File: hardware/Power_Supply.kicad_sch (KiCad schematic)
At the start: 62 parts, among them IC1 LM13700, IC2 LM13700, IC3 LM13700, J5 USB_B, SW1 POWER, U1 TL064, U19 TL064

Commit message: hardware: LCSC review, production files ok
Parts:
- PS1: LCSC C5198614 -> C512062
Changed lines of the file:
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@@
 			)
 		)
-		(property "LCSC" "C5198614"
+		(property "LCSC" "C512062"
 			(at 82.55 76.2 0)
 			(effects

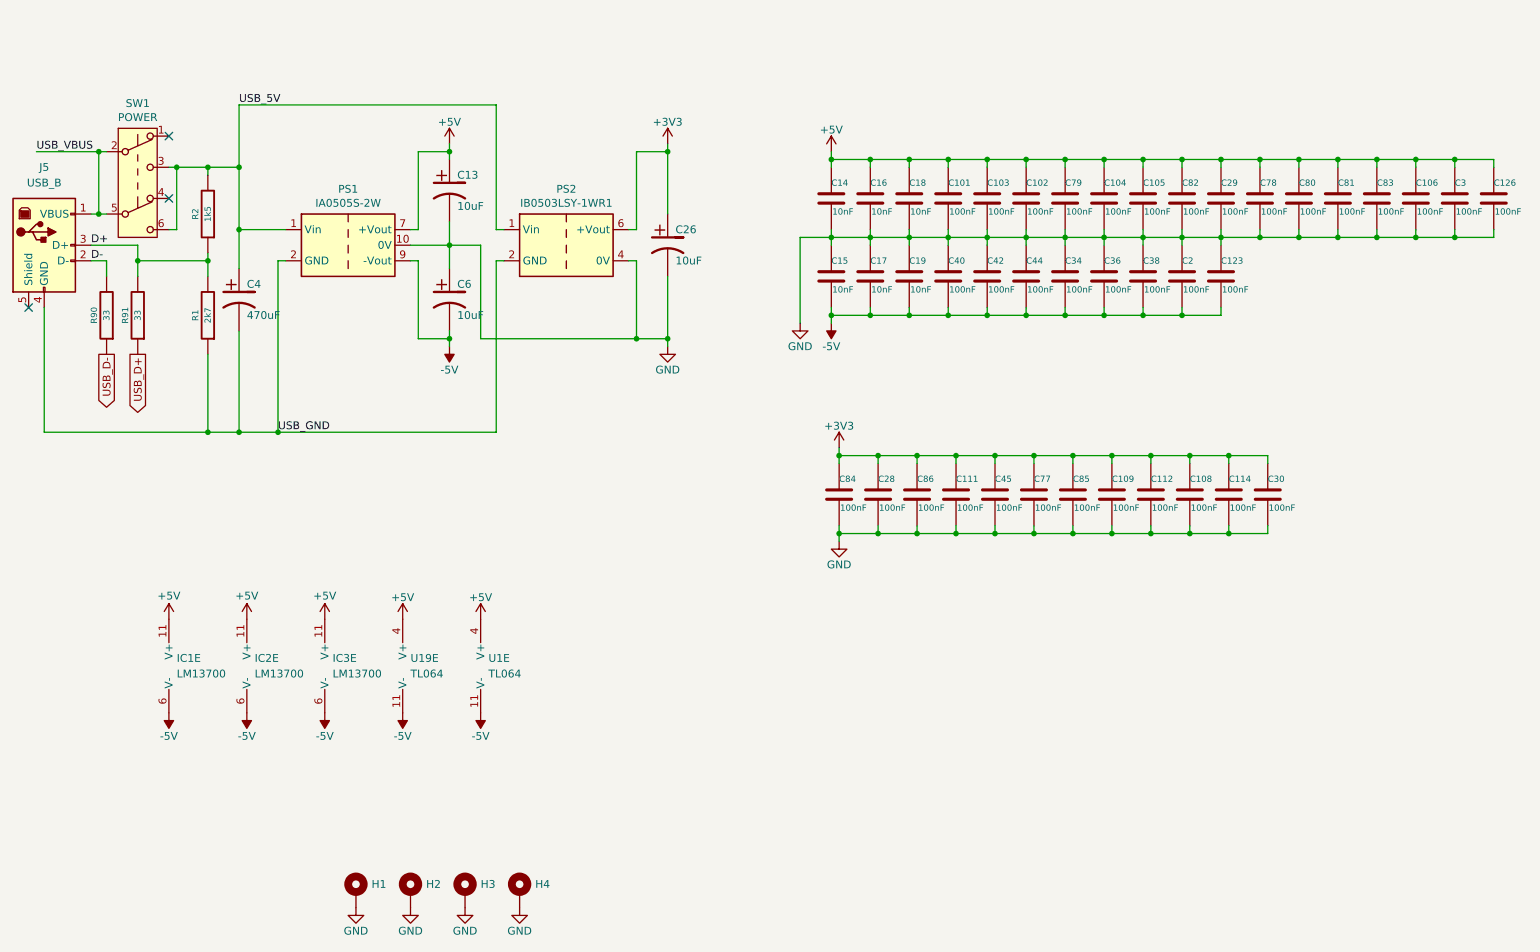
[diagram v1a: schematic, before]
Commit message: hardware: sch/pcb changes by Guimli (adding USB isolator, misc fixes)
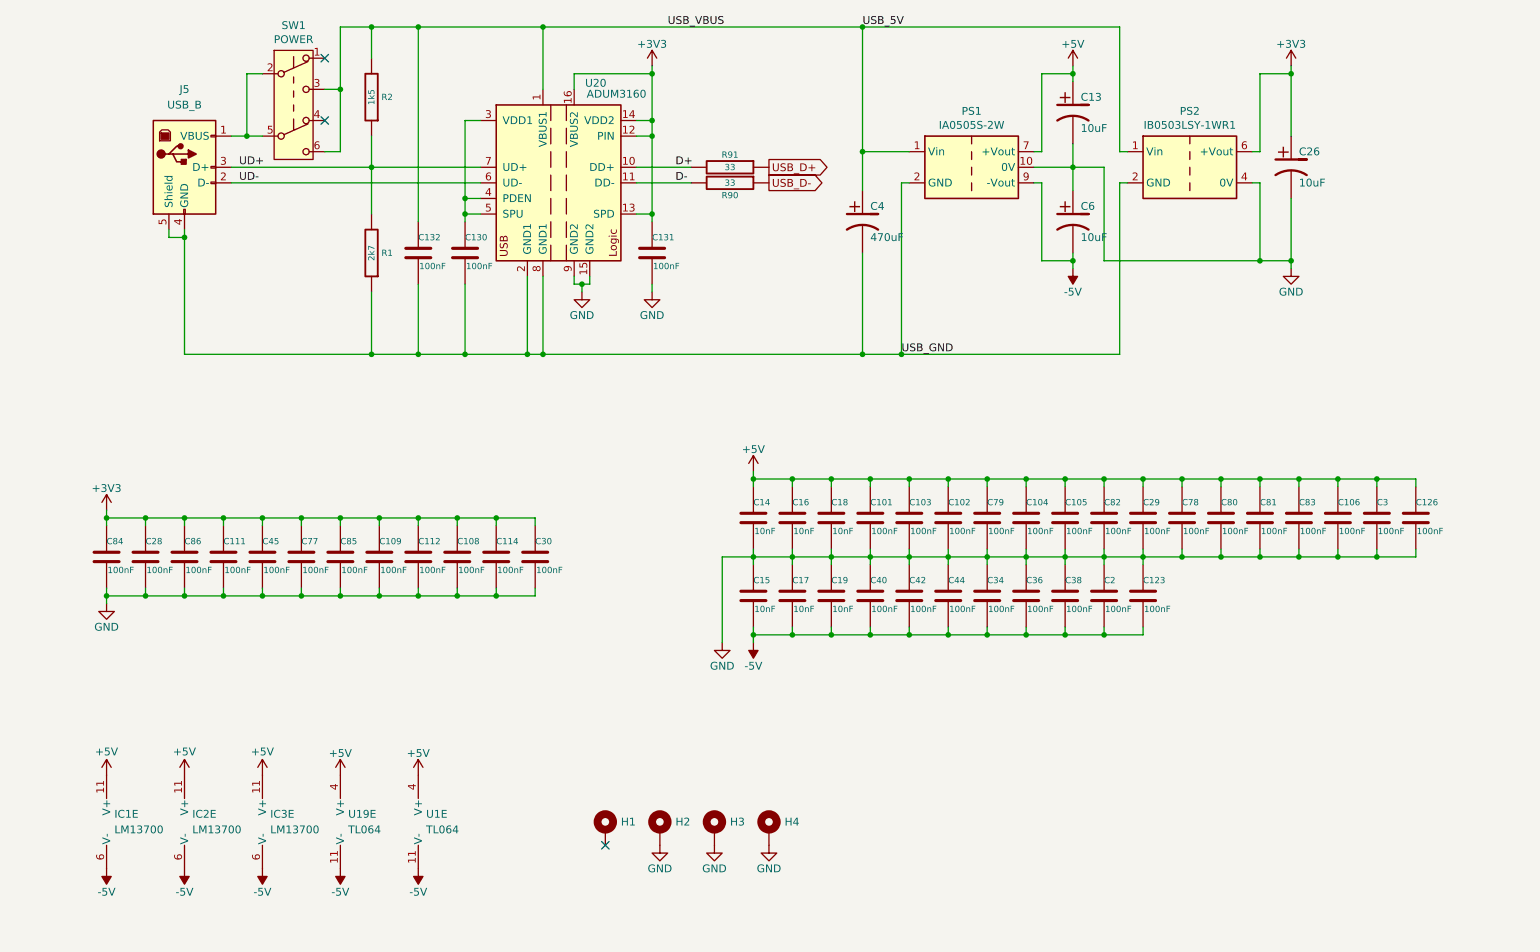
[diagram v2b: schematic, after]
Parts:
- added C130, C131, C132: 100nF, Capacitor_SMD:C_0805_2012Metric, symbol Additional:C
- added U20: ADUM3160, Package_SO:SOIC-16W_7.5x10.3mm_P1.27mm, symbol Interface_USB:ADUM3160
- C13, C26, C6: footprint Capacitor_Tantalum_SMD:CP_EIA-3216-18_Kemet-A -> Additional:CP_EIA-3216-18_Kemet-A
- C4: footprint Capacitor_Tantalum_SMD:CP_EIA-7343-43_Kemet-X -> Additional:CP_EIA-7343-43_Kemet-X
- PS1: LCSC C512062 -> C5198614
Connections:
- net +3V3: now also C131.1, U20.12 (PIN), U20.13 (SPD), U20.14 (VDD2), U20.16 (VBUS2)
- net D+: now also U20.10 (DD+); no longer J5.3 (D+), R1.2, R2.1
- net D-: now also U20.11 (DD-); no longer J5.2 (D-)
- net GND: now also C131.2, U20.15 (GND2), U20.9 (GND2); no longer H1.1
- net USB_5V: now also C132.1, U20.1 (VBUS1)
- net USB_GND: now also J5.5 (Shield), C130.2, C132.2, U20.2 (GND1), U20.8 (GND1)
- net USB_VBUS: no longer names the net of J5.1 (VBUS), SW1.2 (B), SW1.5 (B)
- new net: C130.1, U20.3 (VDD1), U20.4 (PDEN), U20.5 (SPU)
- new net UD+: J5.3 (D+), R1.2, R2.1, U20.7 (UD+)
- new net UD-: J5.2 (D-), U20.6 (UD-)
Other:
- moved on the sheet: C101, C102, C103, C104, C105, C106, C108, C109, C111, C112, C114, C123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

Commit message: hwarware: IA0505S-2W, JETEKPS -> RLT
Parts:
- PS1: LCSC C5198614 -> C512062; Manufacturer JETEKPS -> RLT
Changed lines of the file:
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@@
 			)
 		)
-		(property "Datasheet" "https://www.lcsc.com/datasheet/lcsc_datasheet_2210141730_JETEKPS-IA0505S-2W_C5198614.pdf"
+		(property "Datasheet" "https://wmsc.lcsc.com/wmsc/upload/file/pdf/v2/lcsc/2004151709_rlt-IA0505S-2W_C512062.pdf"
 			(at 173.99 58.42 0)
 			(effects
@@
 			)
 		)
-		(property "Manufacturer" "JETEKPS"
+		(property "Manufacturer" "RLT"
 			(at 184.15 60.96 0)
 			(effects
@@
 			)
 		)
-		(property "LCSC" "C5198614"
+		(property "LCSC" "C512062"
 			(at 184.15 63.5 0)
 			(effects
